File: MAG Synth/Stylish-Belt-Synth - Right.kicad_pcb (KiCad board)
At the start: 2 copper layers, 88.9 x 101.7 mm, 28 parts, among them J1 Amp Board, SW1 Power, U1 stm32f103c8t6-module-china_smd, U2 XPT8871

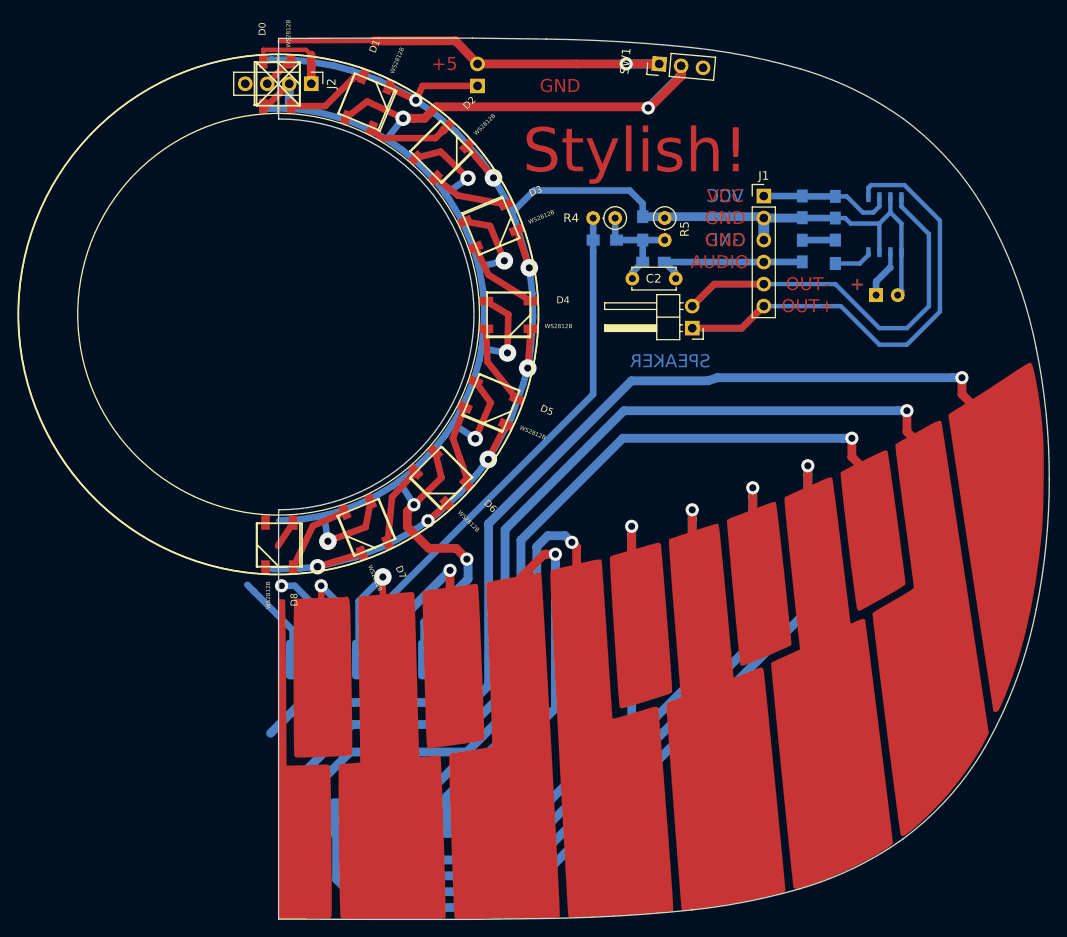
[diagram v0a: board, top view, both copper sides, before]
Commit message: Latest
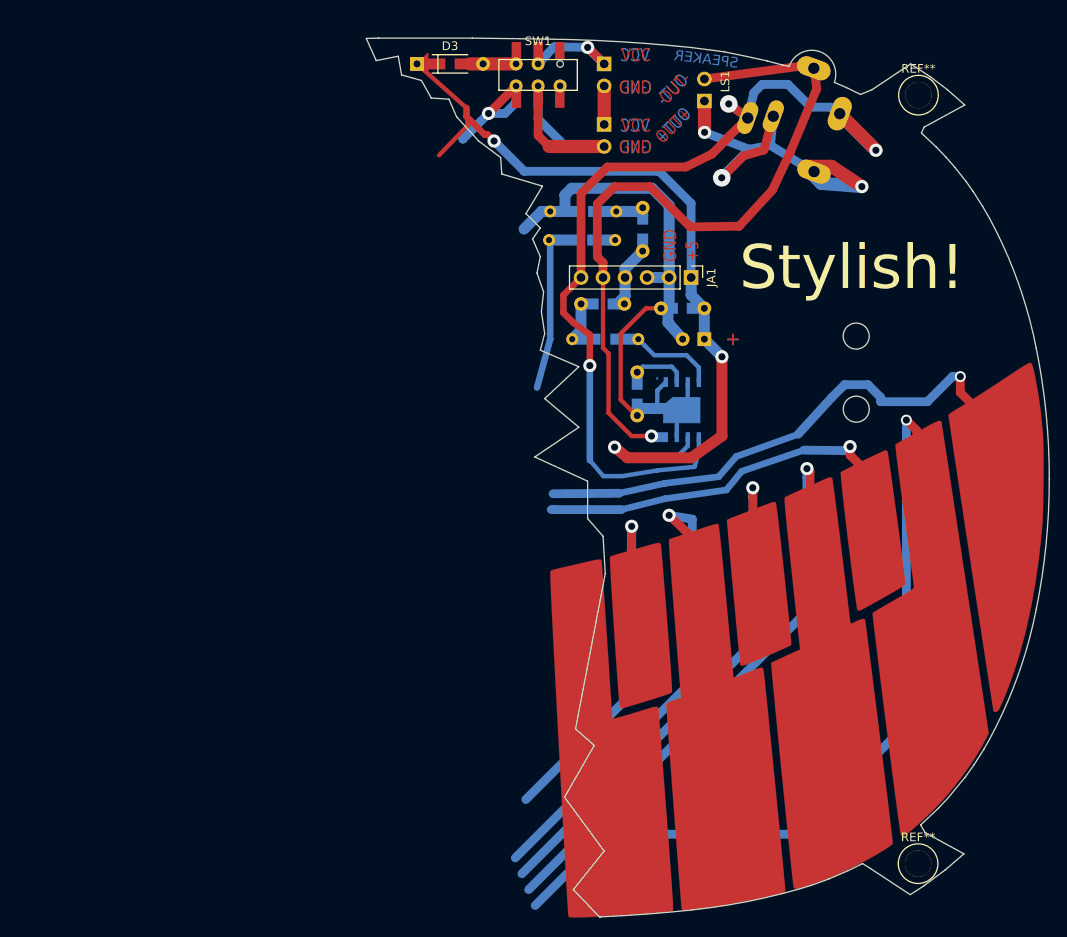
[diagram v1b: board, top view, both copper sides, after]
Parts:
- removed C2: 1uF, Capacitors_ThroughHole:C_Disc_D5.0mm_W2.5mm_P5.00mm
- removed C4: 470uF, Capacitors_SMD:C_0805_HandSoldering
- removed C5: 1uF, Capacitors_SMD:C_0805_HandSoldering
- removed C6: 1uF, Capacitors_ThroughHole:CP_Radial_Tantal_D4.5mm_P2.50mm
- removed C7: 0.39uF, Capacitors_SMD:C_0805_HandSoldering
- removed D0, D1, D2, D4, D5, D6, D7, D8: WS2812B, WS2812B
- removed J2: ~, Pin_Headers:Pin_Header_Straight_1x04_Pitch2.54mm
- removed R4: 10k, Resistors_ThroughHole:R_Axial_DIN0207_L6.3mm_D2.5mm_P2.54mm_Vertical
- removed R5: 1k, Resistors_ThroughHole:R_Axial_DIN0207_L6.3mm_D2.5mm_P2.54mm_Vertical
- removed U1: stm32f103c8t6-module-china_smd, SoftEggKiCAD:stm32f103c8t6-module-china-smd
- added BT1: 4 x 1.5V, Pin_Headers:Pin_Header_Straight_1x02_Pitch2.54mm, B.Cu at (186.1, 57.1)
- added CA1: 470μF, Capacitors_ThroughHole:CP_Radial_Tantal_D4.5mm_P2.50mm, B.Cu at (197.6, 88.9)
- added CA2: 1μF, SoftEggKiCAD:C_Disc_D5.0mm_W2.5mm_P5.00mm+SMD, B.Cu at (197.6, 85.3)
- added CA3: 1μF, SoftEggKiCAD:C_Disc_D5.0mm_W2.5mm_P5.00mm+SMD, B.Cu at (189.9, 92.7)
- added CA4: 0.39μF, SoftEggKiCAD:C_Disc_D5.0mm_W2.5mm_P5.00mm+SMD, B.Cu at (183.4, 84.8)
- added JA1: Conn_01x06, Pin_Headers:Pin_Header_Straight_1x06_Pitch2.54mm, F.Cu at (196.1, 81.8)
- added REF**: AA Battery Holder, SoftEggKiCAD:AA_Battery_Holder_SoftEgg, B.Cu at (215.1, 104.8)
- added REF**: 1pin, Connect:1pin, F.Cu at (222.3, 60.8)
- added REF**: 1pin, Connect:1pin, F.Cu at (222.3, 149.4)
- BT2: footprint Pin_Headers:Pin_Header_Angled_1x02_Pitch2.54mm -> Pin_Headers:Pin_Header_Straight_1x02_Pitch2.54mm
- C1: value 1uF -> 1μF; footprint Capacitors_SMD:C_0805_HandSoldering -> SoftEggKiCAD:C_Disc_D5.0mm_W2.5mm_P5.00mm+SMD
- D3: value WS2812B -> 1N5822; footprint WS2812B -> SoftEggKiCAD:D_DO-35_SOD27_P7.62mm_Horizontal+SMD
- J1: value Amp Board -> Audio-Jack-3_2Switches; footprint Pin_Headers:Pin_Header_Straight_1x06_Pitch2.54mm -> Connectors:Stereo_Jack_3.5mm_Switch_Ledino_KB3SPRS; moved to B.Cu
- KB1: footprint SoftEggKiCAD:MAGWestSynthContactKeybedRight -> SoftEggKiCAD:MAGWestSynthContactKeybed
- LS1: footprint Pin_Headers:Pin_Header_Angled_1x02_Pitch2.54mm -> Pin_Headers:Pin_Header_Straight_1x02_Pitch2.54mm; moved to B.Cu
- R1: value 10k -> 10kΩ; footprint Resistors_SMD:R_0805_HandSoldering -> SoftEggKiCAD:R_Axial_DIN0204_L3.6mm_D1.6mm_P7.62mm_Horizontal+SMD804
- R2: footprint Resistors_SMD:R_0805_HandSoldering -> SoftEggKiCAD:R_Axial_DIN0204_L3.6mm_D1.6mm_P7.62mm_Horizontal+SMD804
- R3: value R -> 100Ω; footprint Resistors_SMD:R_0805_HandSoldering -> SoftEggKiCAD:R_Axial_DIN0204_L3.6mm_D1.6mm_P7.62mm_Horizontal+SMD804
- SW1: footprint Pin_Headers:Pin_Header_Straight_1x03_Pitch2.54mm -> SoftEggKiCAD:MSS22D18+THT
- moved U2 31.6 mm to (195.1, 97.0), turned to 0 degrees
- moved LS1 26.2 mm to (197.6, 61.4), turned to 0 degrees
- moved R3 24.9 mm to (190.0, 88.9), turned to 180 degrees
- moved D3 20.5 mm to (164.5, 57.1), turned to 0 degrees
- moved BT2 15.3 mm to (186.1, 64.1), turned to 180 degrees
- moved SW1 14.0 mm to (178.4, 58.4), turned to 0 degrees
- moved J1 12.9 mm to (213.2, 62.9), turned to 250 degrees
- moved R2 10.8 mm to (179.8, 74.2), turned to 0 degrees
- moved C1 1.78 mm to (190.5, 78.7), turned to 90 degrees
- moved R1 1.19 mm to (187.3, 77.5)
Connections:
- net Net-(KB1-Pad17) renamed /F1
- net Net-(KB1-Pad18) renamed /F#1
- net Net-(KB1-Pad19) renamed /G1
- net Net-(KB1-Pad20) renamed /G#1
- net Net-(KB1-Pad21) renamed /A1
- net Net-(KB1-Pad22) renamed /A#1
- net Net-(KB1-Pad23) renamed /B1
- net Net-(KB1-Pad24) renamed /C2
- BT2 pad 1: /WS2812B-16-LED-RING/GND -> Net-(BT1-Pad2)
- BT2 pad 2: Net-(BT1-Pad1) -> Net-(BT2-Pad2)
- C1 pad 1: /PWM_Audio_Out -> /PWM_OUT
- D3 pad 1: /WS2812B-16-LED-RING/5V -> /+5V
- J1 pad 1: /XH-M125-amp-board/VCC -> /XH-M125-amp-board/OUT+
- J1 pad 2: /WS2812B-16-LED-RING/GND -> /XH-M125-amp-board/OUT+
- J1 pad 3: /WS2812B-16-LED-RING/GND -> /XH-M125-amp-board/OUT-
- J1 pad 4: /PWM_Audio_Out -> Net-(J1-Pad4)
- J1 pad 5: /XH-M125-amp-board/OUT- -> Net-(J1-Pad4)
- LS1 pad 1: /XH-M125-amp-board/OUT+ -> Net-(J1-Pad4)
- R1 pad 2: AUDIO_OUT -> /AUDIO_OUT
- R2 pad 1: /WS2812B-16-LED-RING/GND -> GND
- U2 pad 1: /WS2812B-16-LED-RING/GND -> GND
- U2 pad 3: /WS2812B-16-LED-RING/GND -> GND
- U2 pad 6: /XH-M125-amp-board/VCC -> /+5V
- U2 pad 7: /WS2812B-16-LED-RING/GND -> GND
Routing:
- net /WS2812B-16-LED-RING/5V: track 228.2 -> 0.00 mm, vias 9 -> 0
- net /WS2812B-16-LED-RING/GND: track 202.2 -> 0.00 mm, vias 7 -> 0
- net /+5V: track 0.00 -> 97.7 mm, vias 0 -> 3
- net GND: track 0.00 -> 83.3 mm, vias 0 -> 1
- net AUDIO_OUT: track 62.7 -> 0.00 mm
- net /A#1: track 95.6 -> 39.6 mm
- net /C2: track 111.6 -> 57.7 mm
- net Net-(J1-Pad4): track 0.00 -> 52.6 mm, vias 0 -> 3
- net /F1: track 45.2 -> 0.00 mm, vias 1 -> 0
- net Net-(KB1-Pad16): track 42.0 -> 0.00 mm, vias 1 -> 0
- net /XH-M125-amp-board/OUT+: track 64.0 -> 104.1 mm, vias 0 -> 3
- net Net-(BT1-Pad1): track 48.8 -> 14.7 mm
- net /A1: track 98.4 -> 65.0 mm
- net /XH-M125-amp-board/OUT-: track 54.7 -> 84.7 mm, vias 0 -> 1
- net /G#1: track 87.4 -> 59.2 mm
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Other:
- board size 88.9 x 101.7 mm -> 78.8 x 101.4 mm
- net class Default: trace_width 0.508 -> 0.2
- board text added: "."
- board text added: "MODE"
- board text added: "PATCH"
- board text added: "VALUE"
- board text added: "WRITE"
- board text removed: "20"
- board text removed: "AUDIO"

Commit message: Moving around the gerbers
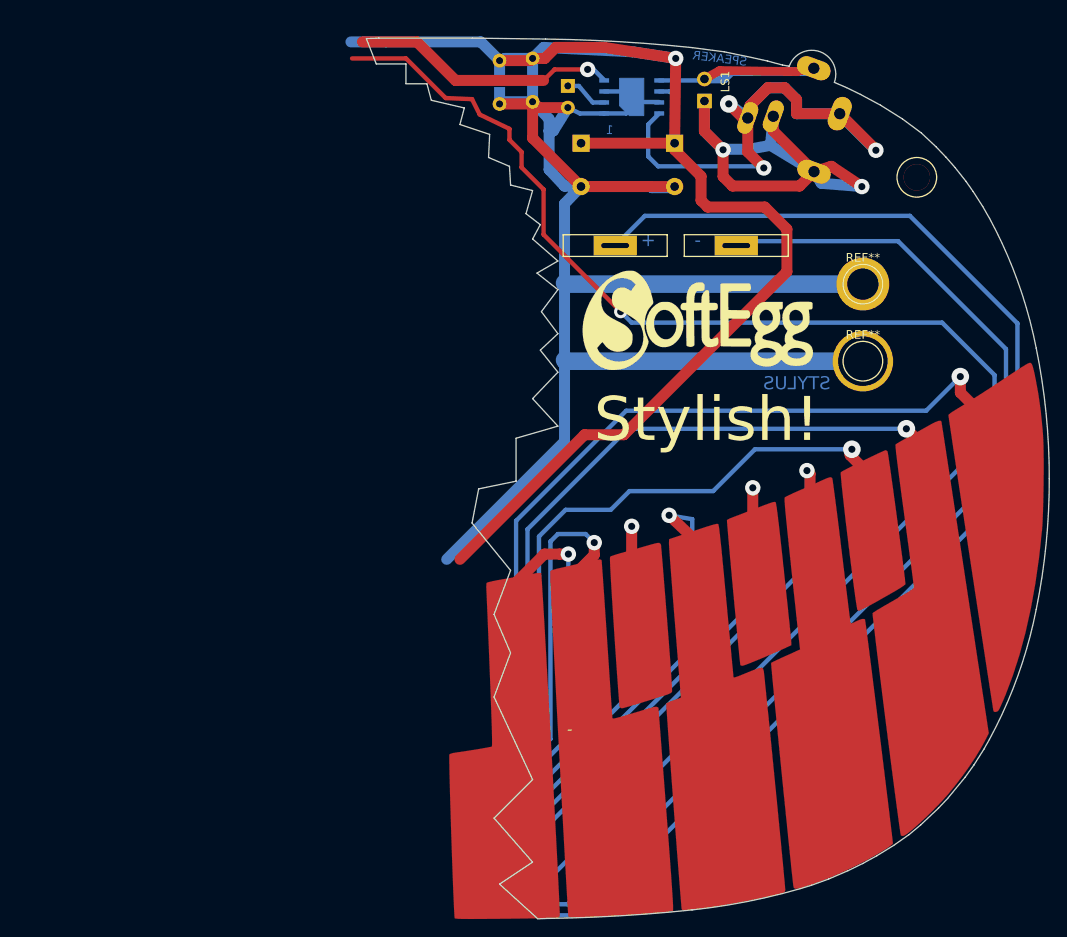
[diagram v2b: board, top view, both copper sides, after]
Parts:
- removed BT1: 4 x 1.5V, Pin_Headers:Pin_Header_Straight_1x02_Pitch2.54mm
- removed BT2: Conn_01x02, Pin_Headers:Pin_Header_Straight_1x02_Pitch2.54mm
- removed C1: 1μF, SoftEggKiCAD:C_Disc_D5.0mm_W2.5mm_P5.00mm+SMD
- removed CA4: 0.39μF, SoftEggKiCAD:C_Disc_D5.0mm_W2.5mm_P5.00mm+SMD
- removed D3: 1N5822, SoftEggKiCAD:D_DO-35_SOD27_P7.62mm_Horizontal+SMD
- removed JA1: Conn_01x06, Pin_Headers:Pin_Header_Straight_1x06_Pitch2.54mm
- removed R1: 10kΩ, SoftEggKiCAD:R_Axial_DIN0204_L3.6mm_D1.6mm_P7.62mm_Horizontal+SMD804
- removed R2: 1k, SoftEggKiCAD:R_Axial_DIN0204_L3.6mm_D1.6mm_P7.62mm_Horizontal+SMD804
- removed R3: 100Ω, SoftEggKiCAD:R_Axial_DIN0204_L3.6mm_D1.6mm_P7.62mm_Horizontal+SMD804
- removed the REF** at (215.1, 104.8)
- removed the REF** at (222.3, 60.8)
- removed the REF** at (222.3, 149.4)
- removed SW1: Power, SoftEggKiCAD:MSS22D18+THT
- added ?: 1pin, Connect:1pin, F.Cu at (222.1, 70.2)
- added BT34: ~, SoftEggKiCAD:AA_Battery_Dual_Terminal, B.Cu at (187.3, 134.0)
- added BTN3: -, SoftEggKiCAD:AA_Battery_-_Terminal, B.Cu at (201.3, 78.1)
- added BTP4: +, SoftEggKiCAD:AA_Battery_+_Terminal, B.Cu at (187.3, 78.1)
- added C2: 1000μF, Capacitors_ThroughHole:CP_Radial_D10.0mm_P5.00mm, B.Cu at (194.2, 66.3)
- added C3: 470μF, Capacitors_ThroughHole:CP_Radial_D10.0mm_P5.00mm, B.Cu at (183.4, 66.3)
- added G***: LOGO, SoftEggKiCAD:SOFTEGG_LOGO2, F.Cu at (196.8, 86.7)
- added REF**: 1pin, Connectors:1pin, F.Cu at (215.9, 82.5)
- added REF**: 1pin, Connectors:1pin, F.Cu at (215.9, 91.4)
- CA1: footprint Capacitors_ThroughHole:CP_Radial_Tantal_D4.5mm_P2.50mm -> SoftEggKiCAD:C_Disc_D5.0mm_W2.5mm_P5.00mm+SMD
- CA3: footprint SoftEggKiCAD:C_Disc_D5.0mm_W2.5mm_P5.00mm+SMD -> Capacitors_ThroughHole:CP_Radial_Tantal_D4.5mm_P2.50mm
- J1: value Audio-Jack-3_2Switches -> Headphone
- KB1: footprint SoftEggKiCAD:MAGWestSynthContactKeybed -> SoftEggKiCAD:MAGWestSynthContactKeybedRight2
- LS1: value SPEAKER -> Speaker
- moved CA1 39.9 mm to (174.0, 56.8), turned to 270 degrees
- moved U2 36.5 mm to (189.2, 61.0), turned to 90 degrees
- moved CA2 35.0 mm to (177.8, 56.5), turned to 270 degrees
- moved CA3 34.0 mm to (181.9, 59.7)
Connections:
- J1 pad 1: /XH-M125-amp-board/OUT+ -> Net-(J1-Pad1)
- J1 pad 2: /XH-M125-amp-board/OUT+ -> Net-(J1-Pad1)
- J1 pad 3: /XH-M125-amp-board/OUT- -> Net-(J1-Pad3)
- LS1 pad 2: /XH-M125-amp-board/OUT- -> Net-(J1-Pad3)
- U2 pad 5: /XH-M125-amp-board/OUT+ -> Net-(J1-Pad3)
- U2 pad 8: /XH-M125-amp-board/OUT- -> Net-(J1-Pad1)
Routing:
- net /LED_DIN: track 0.00 -> 179.2 mm, vias 0 -> 1
- net Net-(BTP4-Pad1): track 0.00 -> 150.4 mm
- net Net-(BTN3-Pad1): track 0.00 -> 127.9 mm
- net GND: track 83.3 -> 196.6 mm, vias 1 -> 0
- net /XH-M125-amp-board/OUT+: track 104.1 -> 0.00 mm, vias 3 -> 0
- net /XH-M125-amp-board/OUT-: track 84.7 -> 0.00 mm, vias 1 -> 0
- net Net-(J1-Pad1): track 0.00 -> 77.0 mm, vias 0 -> 3
- net /+5V: track 97.7 -> 163.6 mm, vias 3 -> 1
- net /F1: track 0.00 -> 39.2 mm, vias 0 -> 1
- net /E1: track 0.00 -> 37.5 mm, vias 0 -> 1
- net /A#1: track 39.6 -> 71.3 mm
- net /C2: track 57.7 -> 89.0 mm
- net Net-(J1-Pad3): track 0.00 -> 31.1 mm
- net Net-(BT2-Pad2): track 26.6 -> 0.00 mm
- net Net-(RA1-Pad1): track 10.0 -> 30.8 mm, vias 0 -> 1
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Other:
- board size 78.8 x 101.4 mm -> 78.8 x 101.6 mm
- net class Default: trace_width 0.2 -> 0.635; via_dia 2.032 -> 1.524
- board text added: "-"
- board text added: "1"
- board text added: "STYLUS"
- board text removed: "+5"
- board text removed: "."
- board text removed: "GND"
- board text removed: "MODE"
- board text removed: "OUT+"
- board text removed: "OUT-"
- board text removed: "PATCH"
- board text removed: "VALUE"
- board text removed: "VCC"
- board text removed: "WRITE"
